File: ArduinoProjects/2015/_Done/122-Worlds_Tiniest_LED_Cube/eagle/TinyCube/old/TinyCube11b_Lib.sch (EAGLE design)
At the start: 18 parts

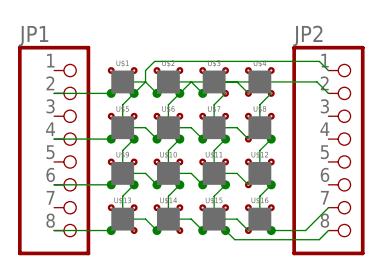
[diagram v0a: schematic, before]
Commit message: folder cleanup
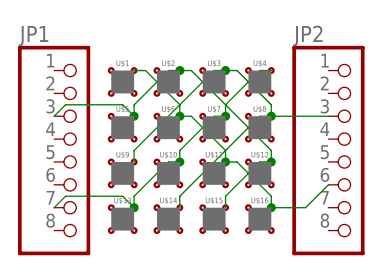
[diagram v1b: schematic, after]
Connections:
- removed net N$5: JP2.1, U$1.R, U$13.R, U$5.R, U$9.R
- removed net N$6: JP2.7, U$12.R, U$16.R, U$4.R, U$8.R
- removed net N$7: JP2.8, U$11.R, U$15.R, U$3.R, U$7.R
- removed net N$8: JP2.2, U$10.R, U$14.R, U$2.R, U$6.R
- net N$1: now also JP1.3, U$12.G, U$15.G, U$2.G, U$5.G; no longer JP1.2, U$1.A, U$2.A, U$3.A, U$4.A
- net N$2: now also JP1.7, U$10.G, U$13.G, U$4.G, U$7.G; no longer JP1.4, U$5.A, U$6.A, U$7.A, U$8.A
- net N$3: now also JP2.6, U$1.G, U$11.G, U$16.G, U$6.G; no longer JP1.6, U$10.A, U$11.A, U$12.A, U$9.A
- net N$4: now also JP2.3, U$14.G, U$3.G, U$8.G, U$9.G; no longer JP1.8, U$13.A, U$14.A, U$15.A, U$16.A
